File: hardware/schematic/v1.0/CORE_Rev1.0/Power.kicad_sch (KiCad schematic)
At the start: 26 parts, among them CN1 LAIL-PHC2_54-2P-01-XH-L, J10 USB_C_Receptacle_USB2.0_16P, U2 TPS78633, U5 AMS1117-1.8

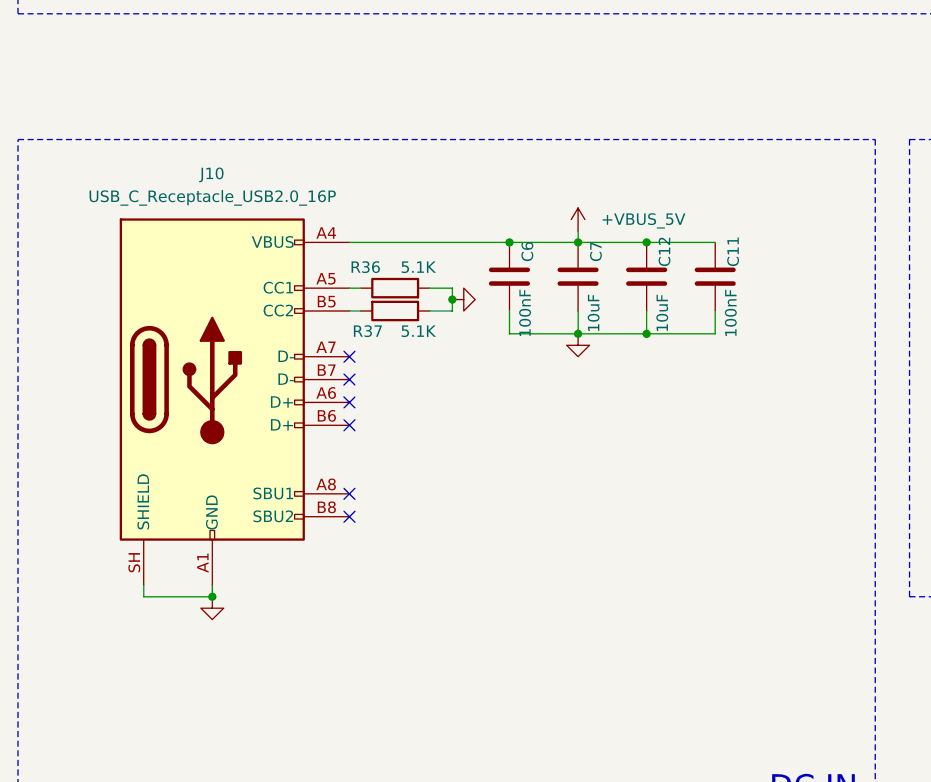
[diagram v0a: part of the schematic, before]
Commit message: sch update
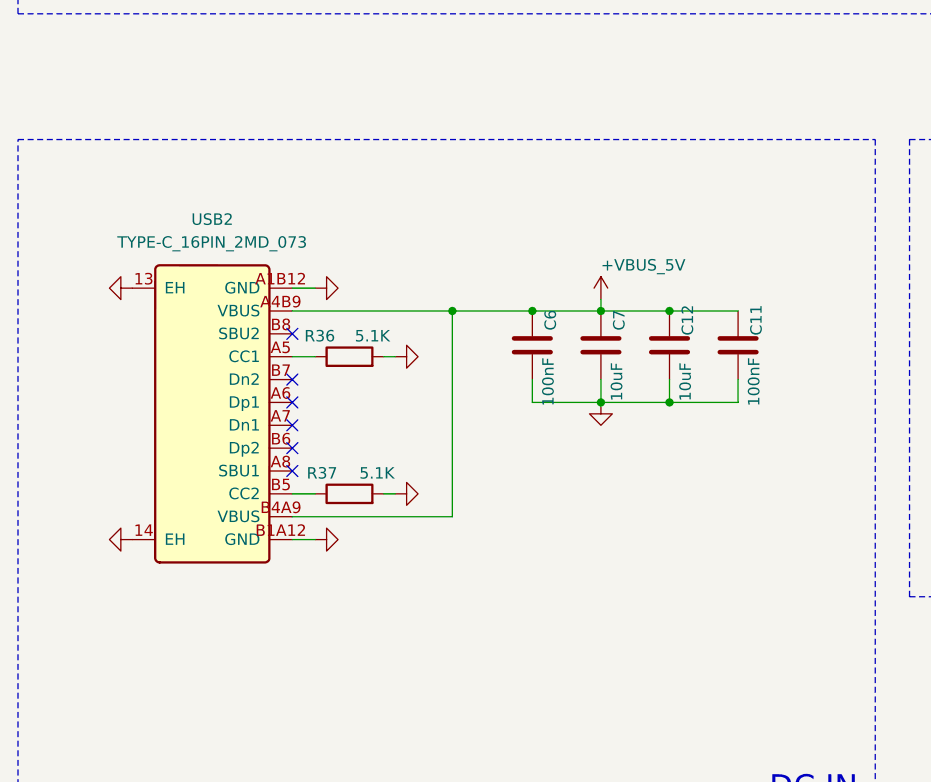
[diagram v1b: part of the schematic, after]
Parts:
- removed J10: USB_C_Receptacle_USB2.0_16P, Connector_USB:USB_C_Receptacle_Palconn_UTC16-G, symbol Connector:USB_C_Receptacle_USB2.0_16P
- added USB2: TYPE-C_16PIN_2MD_073, CORE:TYPE-C_16PIN_2MD_073, symbol CORE:TYPE-C_16PIN_2MD_073
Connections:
- net +VBUS_5V: now also USB2.A4B9 (VBUS), USB2.B4A9 (VBUS)
- net GND: now also R37.2, USB2.13 (EH), USB2.14 (EH), USB2.A1B12 (GND), USB2.B1A12 (GND); no longer R37.1
- net at R36.1: now also USB2.A5 (CC1)
- new net: R37.1, USB2.B5 (CC2)
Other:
- moved on the sheet: C11, C12, C6, C7, R36

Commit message: sch update
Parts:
- C10, C12, C15, C16, C17, C18, C26, C7, C8: footprint Capacitor_SMD:C_0603_1608Metric -> CORE:C_0603_1608Metric; symbol Device:C -> CORE:C
- C11, C19, C27, C6, C9: footprint Capacitor_SMD:C_0402_1005Metric -> CORE:C_0402_1005Metric; symbol Device:C -> CORE:C
- D7: footprint LED_SMD:LED_0603_1608Metric -> CORE:LED_0603_1608Metric; symbol Device:LED -> CORE:LED
- R36, R37, R40, R45: footprint Resistor_SMD:R_0402_1005Metric -> CORE:R_0402_1005Metric; symbol Device:R -> CORE:R
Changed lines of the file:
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@@
 	)
 	(symbol
-		(lib_id "Device:C")
+		(lib_id "CORE:C")
 		(at 76.2 101.6 0)
 		(unit 1)
@@
 			)
 		)
-		(property "Footprint" "Capacitor_SMD:C_0402_1005Metric"
+		(property "Footprint" "CORE:C_0402_1005Metric"
 			(at 77.1652 105.41 0)
 			(hide yes)
@@
 	)
 	(symbol
-		(lib_id "Device:R")
+		(lib_id "CORE:R")
 		(at 55.88 102.87 90)
 		(unit 1)
@@
 			)
 		)
-		(property "Footprint" "Resistor_SMD:R_0402_1005Metric"
+		(property "Footprint" "CORE:R_0402_1005Metric"
 			(at 55.88 104.648 90)
 			(hide yes)
@@
 	)
 	(symbol
-		(lib_id "Device:C")
+		(lib_id "CORE:C")
 		(at 29.21 45.72 180)
 		(unit 1)
@@
 			)
 		)
-		(property "Footprint" "Capacitor_SMD:C_0603_1608Metric"
+		(property "Footprint" "CORE:C_0603_1608Metric"
 			(at 28.2448 41.91 0)
 			(hide yes)
@@
 	)
 	(symbol
-		(lib_id "Device:LED")
+		(lib_id "CORE:LED")
 		(at 213.36 114.3 90)
 		(unit 1)
@@
 			)
 		)
-		(property "Footprint" "LED_SMD:LED_0603_1608Metric"
+		(property "Footprint" "CORE:LED_0603_1608Metric"
 			(at 213.36 114.3 0)
 			(hide yes)
@@
 	)
 	(symbol
-		(lib_id "Device:C")
+		(lib_id "CORE:C")
 		(at 92.71 39.37 0)
 		(unit 1)
@@
 			)
 		)
-		(property "Footprint" "Capacitor_SMD:C_0603_1608Metric"
+		(property "Footprint" "CORE:C_0603_1608Metric"
 			(at 93.6752 43.18 0)
 			(hide yes)
@@
 	)
 	(symbol
-		(lib_id "Device:C")
+		(lib_id "CORE:C")
 		(at 100.33 39.37 0)
 		(unit 1)
@@
 			)
 		)
-		(property "Footprint" "Capacitor_SMD:C_0603_1608Metric"
+		(property "Footprint" "CORE:C_0603_1608Metric"
 			(at 101.2952 43.18 0)
 			(hide yes)
@@
 	)
 	(symbol
-		(lib_id "Device:R")
+		(lib_id "CORE:R")
 		(at 213.36 105.41 0)
 		(unit 1)
@@
 			)
 		)
-		(property "Footprint" "Resistor_SMD:R_0402_1005Metric"
+		(property "Footprint" "CORE:R_0402_1005Metric"
 			(at 211.582 105.41 90)
 			(hide yes)
@@
 	)
 	(symbol
-		(lib_id "Device:R")
+		(lib_id "CORE:R")
 		(at 55.88 118.11 90)
 		(unit 1)
@@
 			)
 		)
-		(property "Footprint" "Resistor_SMD:R_0402_1005Metric"
+		(property "Footprint" "CORE:R_0402_1005Metric"
 			(at 55.88 119.888 90)
 			(hide yes)
@@
 	)
 	(symbol
-		(lib_id "Device:C")
+		(lib_id "CORE:C")
 		(at 153.67 102.87 0)
 		(unit 1)
@@
 			)
 		)
-		(property "Footprint" "Capacitor_SMD:C_0402_1005Metric"
+		(property "Footprint" "CORE:C_0402_1005Metric"
 			(at 153.67 102.87 0)
 			(hide yes)
@@
 	)
 	(symbol
-		(lib_id "Device:R")
+		(lib_id "CORE:R")
 		(at 29.21 36.83 180)
 		(unit 1)
@@
 			)
 		)
-		(property "Footprint" "Resistor_SMD:R_0402_1005Metric"
+		(property "Footprint" "CORE:R_0402_1005Metric"
 			(at 30.988 36.83 90)
 			(hide yes)
@@
 	)
 	(symbol
-		(lib_id "Device:C")
+		(lib_id "CORE:C")
 		(at 83.82 101.6 0)
 		(unit 1)
@@
 			)
 		)
-		(property "Footprint" "Capacitor_SMD:C_0603_1608Metric"
+		(property "Footprint" "CORE:C_0603_1608Metric"
 			(at 84.7852 105.41 0)
 			(hide yes)
@@
 	)
 	(symbol
-		(lib_id "Device:C")
+		(lib_id "CORE:C")
 		(at 119.38 39.37 0)
 		(unit 1)
@@
 			)
 		)
-		(property "Footprint" "Capacitor_SMD:C_0603_1608Metric"
+		(property "Footprint" "CORE:C_0603_1608Metric"
 			(at 120.3452 43.18 0)
 			(hide yes)
@@
 	)
 	(symbol
-		(lib_id "Device:C")
+		(lib_id "CORE:C")
 		(at 127 39.37 0)
 		(unit 1)
@@
 			)
 		)
-		(property "Footprint" "Capacitor_SMD:C_0603_1608Metric"
+		(property "Footprint" "CORE:C_0603_1608Metric"
 			(at 127.9652 43.18 0)
 			(hide yes)
@@
 	)
 	(symbol
-		(lib_id "Device:C")
+		(lib_id "CORE:C")
 		(at 99.06 101.6 0)
 		(unit 1)
@@
 			)
 		)
-		(property "Footprint" "Capacitor_SMD:C_0402_1005Metric"
+		(property "Footprint" "CORE:C_0402_1005Metric"
 			(at 100.0252 105.41 0)
 			(hide yes)
@@
 	)
 	(symbol
-		(lib_id "Device:C")
+		(lib_id "CORE:C")
 		(at 91.44 101.6 0)
 		(unit 1)
@@
 			)
 		)
-		(property "Footprint" "Capacitor_SMD:C_0603_1608Metric"
+		(property "Footprint" "CORE:C_0603_1608Metric"
 			(at 92.4052 105.41 0)
 			(hide yes)
@@
 	)
 	(symbol
-		(lib_id "Device:C")
+		(lib_id "CORE:C")
 		(at 72.39 38.1 180)
 		(unit 1)
@@
 			)
 		)
-		(property "Footprint" "Capacitor_SMD:C_0603_1608Metric"
+		(property "Footprint" "CORE:C_0603_1608Metric"
 			(at 71.4248 34.29 0)
 			(hide yes)
@@
 	)
 	(symbol
-		(lib_id "Device:C")
+		(lib_id "CORE:C")
 		(at 57.15 45.72 180)
 		(unit 1)
@@
 			)
 		)
-		(property "Footprint" "Capacitor_SMD:C_0402_1005Metric"
+		(property "Footprint" "CORE:C_0402_1005Metric"
 			(at 56.1848 41.91 0)
 			(hide yes)
@@
 	)
 	(symbol
-		(lib_id "Device:C")
+		(lib_id "CORE:C")
 		(at 63.5 38.1 180)
 		(unit 1)
@@
 			)
 		)
-		(property "Footprint" "Capacitor_SMD:C_0402_1005Metric"
+		(property "Footprint" "CORE:C_0402_1005Metric"
 			(at 62.5348 34.29 0)
 			(hide yes)
@@
 	)
 	(symbol
-		(lib_id "Device:C")
+		(lib_id "CORE:C")
 		(at 146.05 102.87 0)
 		(unit 1)
@@
 			)
 		)
-		(property "Footprint" "Capacitor_SMD:C_0603_1608Metric"
+		(property "Footprint" "CORE:C_0603_1608Metric"
 			(at 146.05 102.87 0)
 			(hide yes)
